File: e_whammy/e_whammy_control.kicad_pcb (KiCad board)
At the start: 2 copper layers, 34 x 14 mm, 33 parts, among them J1 Conn_01x03, J2 Conn_01x03, J3 Conn_01x02, J4 Conn_01x02, U2 HT7550-1, U3 TLV9004IPWR

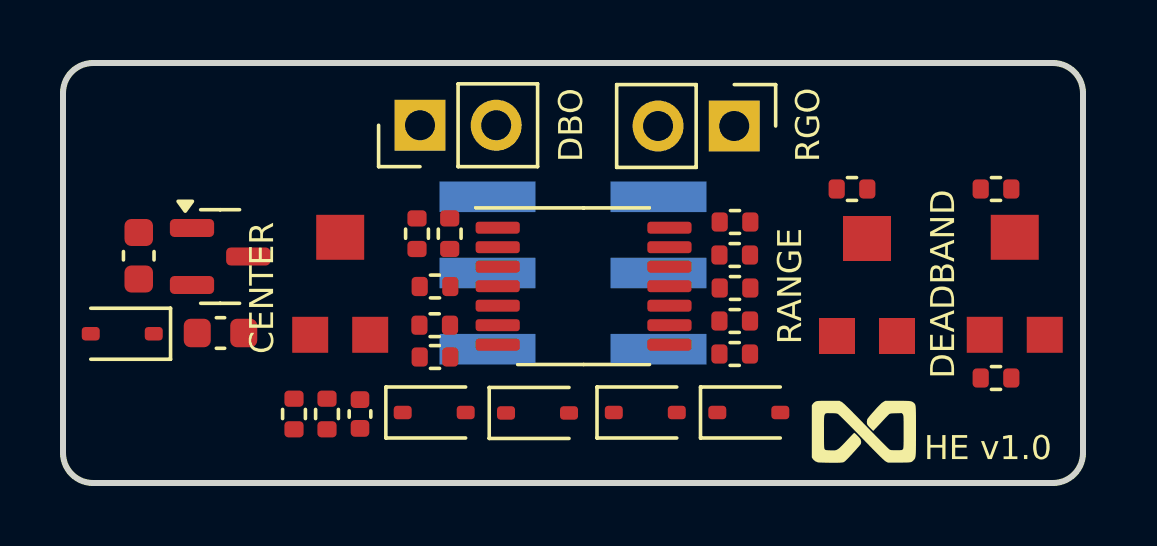
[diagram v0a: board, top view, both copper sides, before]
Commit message: E-Whammy layout complete (first shot)
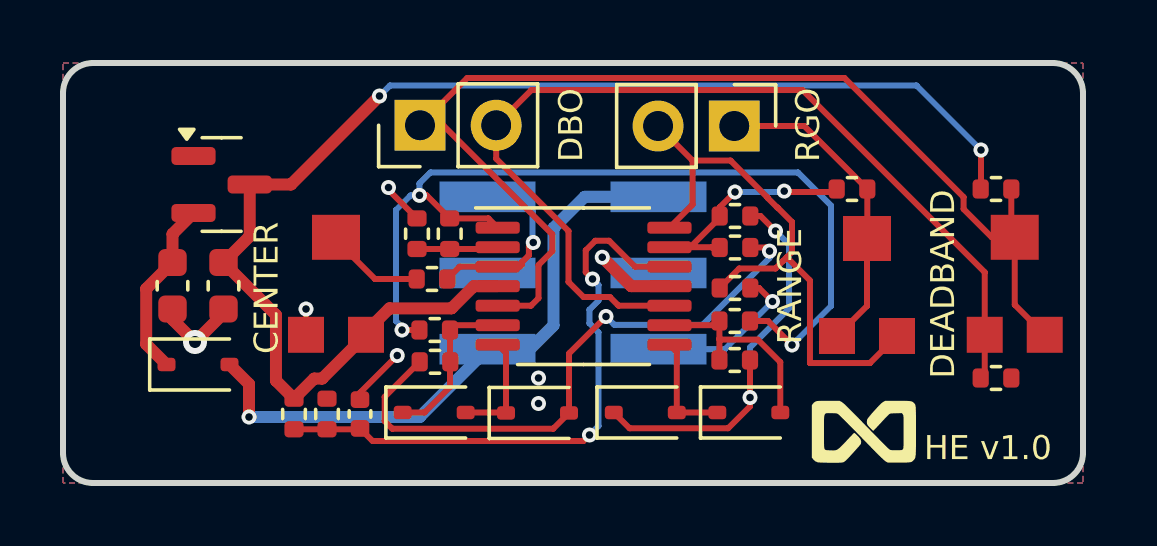
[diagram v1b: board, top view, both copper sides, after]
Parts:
- moved D2 2.73 mm to (139.5, 149.1), turned to 0 degrees
- moved J1 2.54 mm to (149.2, 146.0)
- moved J2 2.54 mm to (154.8, 146.0)
- moved U2 2.40 mm to (140.3, 143.1)
- moved C4 1.58 mm to (140.3, 146.4), turned to -90 degrees
- moved C3 1.51 mm to (138.7, 146.4), turned to -90 degrees
- moved R6 0.27 mm to (147.3, 146.2)
- moved R12 0.25 mm to (157.4, 145.2)
- moved R11 0.20 mm to (157.4, 148.9)
- moved R13 0.20 mm to (157.4, 144.1)
- moved R10 0.16 mm to (147.4, 149.0)
- moved R3 0.16 mm to (147.4, 147.9)
- moved RV1 0.14 mm to (144.1, 146.3)
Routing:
- net 5v: track 0.00 -> 44.8 mm, vias 0 -> 2
- net /DHI: track 0.00 -> 37.9 mm
- net /DLO: track 0.00 -> 32.8 mm
- net /PRE: track 0.00 -> 30.3 mm, vias 0 -> 3
- net V+: track 0.00 -> 20.6 mm, vias 0 -> 1
- net /VREF: track 0.00 -> 20.1 mm, vias 0 -> 2
- net /PR: track 0.00 -> 20.1 mm, vias 0 -> 2
- net /RO2: track 0.00 -> 19.4 mm
- net /NR: track 0.00 -> 13.9 mm, vias 0 -> 2
- net /RO1: track 0.00 -> 10.6 mm
- net GND: track 0.00 -> 9.81 mm, vias 0 -> 7
- net Net-(U3D--): track 0.00 -> 8.29 mm, vias 0 -> 2
- net Net-(D5-A): track 0.00 -> 7.05 mm
- net HE_SENSOR: track 0.00 -> 6.33 mm, vias 0 -> 1
- net Net-(D2-K): track 0.00 -> 5.98 mm
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- added copper zone on B.Cu, net GND
- added copper zone on F.Cu, net GND
